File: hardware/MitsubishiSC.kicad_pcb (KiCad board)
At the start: 6 copper layers, 35 x 50 mm, 68 parts, among them J1 CN105, J2 USB_C_Receptacle_USB2.0_16P, J3 Conn_01x04, Q1 BSS138, Q2 BSS138, SW3 SPST, SW4 SPST, U1 TPS563201, U3 ESP32-C6-WROOM-1, U4 USBLC6-2SC6, U5 TLV75733PDBV

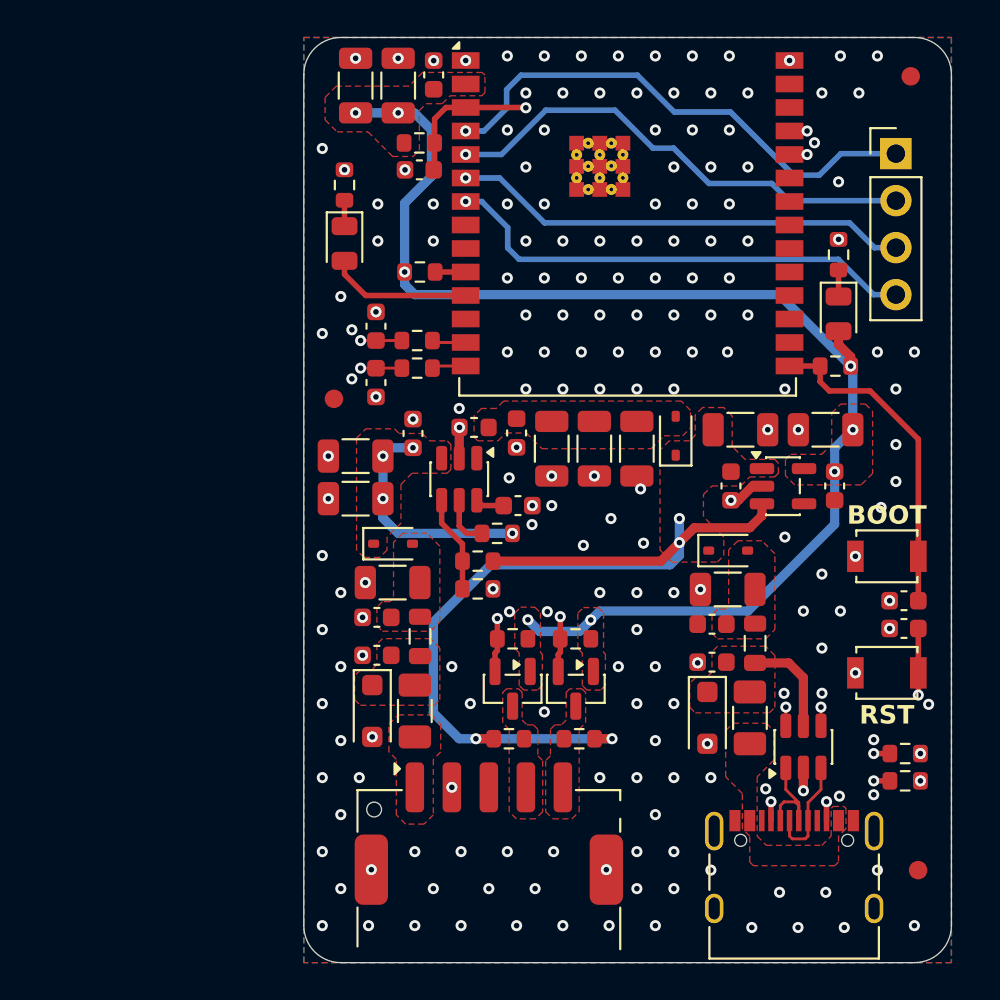
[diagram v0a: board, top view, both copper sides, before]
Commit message: feat: redesign PCB layout (#41)
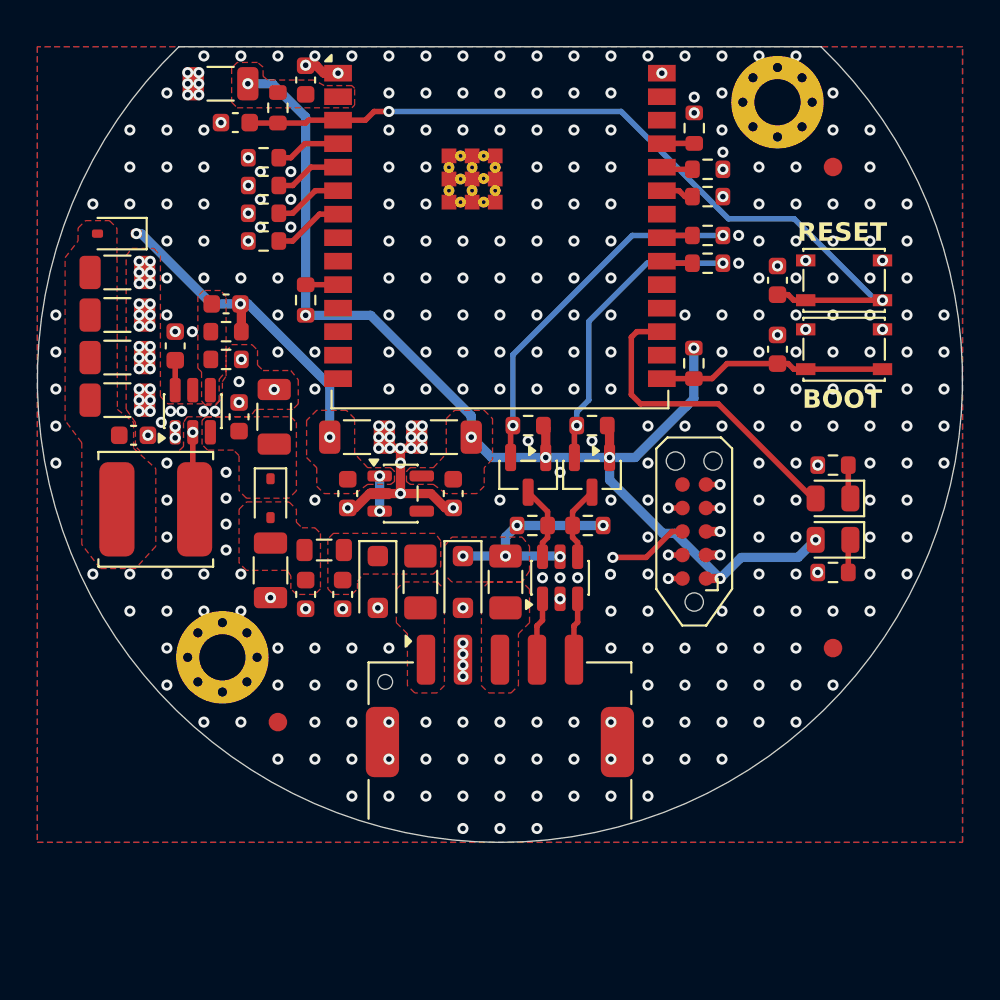
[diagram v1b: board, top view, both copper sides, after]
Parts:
- removed C22: 10uF, Capacitor_SMD:C_1206_3216Metric
- removed C23, C26: 100nF, Capacitor_SMD:C_0603_1608Metric
- removed C24, C25: NC, Capacitor_SMD:C_0603_1608Metric
- removed D7: CUS10S30, Diode_SMD:D_SOD-323
- removed D8: SMF4L5.0A, Diode_SMD:D_SOD-123F
- removed FB2: 220R@100MHz, Inductor_SMD:L_0805_2012Metric
- removed J3: Conn_01x04, Connector_PinHeader_2.54mm:PinHeader_1x04_P2.54mm_Vertical
- removed SW3, SW4: SPST, Button_Switch_SMD:SW_SPST_B3U-1000P
- removed U5: TLV75733PDBV, Package_TO_SOT_SMD:SOT-23-5
- added D6: BU, LED_SMD:LED_0805_2012Metric, F.Cu at (171.1, 104.5)
- added H1: #2, MountingHole:MountingHole_2.5mm_Pad_Via, F.Cu at (168.1, 83.1)
- added H2: #2, MountingHole:MountingHole_2.5mm_Pad_Via, F.Cu at (138.1, 113.1)
- added R17: 10kR, Resistor_SMD:R_0603_1608Metric, F.Cu at (157.8, 106.0)
- added R18: 10kR, Resistor_SMD:R_0603_1608Metric, F.Cu at (158.1, 100.6)
- added R19: 10kR, Resistor_SMD:R_0603_1608Metric, F.Cu at (171.1, 108.5)
- added R20: 10kR, Resistor_SMD:R_0603_1608Metric, F.Cu at (171.1, 102.7)
- added SW1: SPST, Button_Switch_SMD:SW_SPST_PTS810, F.Cu at (171.7, 92.7)
- added SW2: SPST, Button_Switch_SMD:SW_SPST_PTS810, F.Cu at (171.7, 96.5)
- added U2: TPS54202DDC, Package_TO_SOT_SMD:SOT-23-6, F.Cu at (136.5, 99.8)
- C11, C17, C20, C21: value 10uF -> 100nF; footprint Capacitor_SMD:C_1206_3216Metric -> Capacitor_SMD:C_0603_1608Metric
- C13, C14, C15, C19: value 100nF -> 10uF; footprint Capacitor_SMD:C_0603_1608Metric -> Capacitor_SMD:C_1206_3216Metric
- C16: value 10uF -> 68pF; footprint Capacitor_SMD:C_1206_3216Metric -> Capacitor_SMD:C_0603_1608Metric
- D1: value SMF4L12A -> CUS10S30; footprint Diode_SMD:D_SOD-123F -> Diode_SMD:D_SOD-323
- D3: value RED -> SMF4L12A; footprint LED_SMD:LED_0805_2012Metric -> Diode_SMD:D_SOD-123F
- D4: value CUS10S30 -> SMF4L5.0A; footprint Diode_SMD:D_SOD-323 -> Diode_SMD:D_SOD-123F
- D5: value BLUE -> RD
- F2: value 350mA -> 125mA
- J2: value USB_C_Receptacle_USB2.0_16P -> TC2050; footprint Connector_USB:USB_C_Receptacle_XKB_U262-16XN-4BVC11 -> Connector:Tag-Connect_TC2050-IDC-NL_2x05_P1.27mm_Vertical
- L1: value 3.3uH -> 15uH; footprint Inductor_SMD:L_0603_1608Metric -> Inductor_SMD:L_TDK_VLS6045EX_VLS6045AF
- R10: value 54.9kR -> 10kR
- R11, R12, R3, R4, R6: value 10kR -> 0R
- R13: value 10kR -> 100kR
- R14: value 5.1kR -> 13.3kR
- R15: value 5.1kR -> 10kR
- R16: value 22R -> 10kR
- R5: value 10kR -> 470R
- R7: value 22R -> 0R
- R9: value 1kR -> 0R
- U1: value TPS563201 -> ESP32-C6-WROOM-1; footprint Package_TO_SOT_SMD:SOT-23-6 -> _Custom:ESP32-C6-WROOM-1
- U3: value ESP32-C6-WROOM-1 -> TLV75733PDBV; footprint _Custom:ESP32-C6-WROOM-1 -> Package_TO_SOT_SMD:SOT-23-5
- moved FID3 48.9 mm to (141.1, 116.6)
- moved R14 43.2 mm to (138.3, 97.0)
- moved FID2 38.3 mm to (171.1, 86.6)
- moved C14 36.2 mm to (132.4, 94.6), turned to 0 degrees
- moved R3 35.7 mm to (140.3, 86.1), turned to 0 degrees
- moved C19 34.4 mm to (140.7, 108.4), turned to -90 degrees
- moved C4 33.7 mm to (135.6, 96.3), turned to 90 degrees
- moved C18 32.3 mm to (142.6, 109.7), turned to -90 degrees
- moved R1 31.4 mm to (141.1, 83.4), turned to -90 degrees
- moved R9 31.1 mm to (140.3, 90.6), turned to 0 degrees
- moved D5 30.9 mm to (171.1, 106.8), turned to 180 degrees
- moved FID1 30.1 mm to (171.1, 112.6)
- moved R4 29.7 mm to (140.3, 87.6)
- moved D1 29.3 mm to (132.4, 90.2), turned to 180 degrees
- moved D3 28.8 mm to (146.5, 109.0)
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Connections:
- C1 pad 1: +12V -> +3.3V
- C11 pad 1: +3.3V -> /SMPS_SW_5V
- C12 pad 1: +3.3V -> /SMPS_SW_5V
- C13 pad 1: /CN105_12V_FLT -> /SMPS_SW_5V
- C14 pad 1: /USB_5V_D -> /SMPS_SW_5V
- C15 pad 1: /CN105_12V_D -> /SMPS_SW_5V
- C16 pad 1: /SMPS_5V_D -> +5V
- C16 pad 2: GND -> /SMPS_FB
- C17 pad 1: /SMPS_5V_D -> /CN105_12V_FSD
- C18 pad 1: /MCU_BOOT -> /CN105_12V_FLT
- C19 pad 1: /MCU_RST -> /CN105_12V_FLT
- C2 pad 1: /SMPS_5V -> +3.3V
- C2 pad 2: /SMPS_BST -> GND
- C20 pad 1: /CN105_12V_D -> /MCU_RST
- C21 pad 1: /USB_5V_D -> /MCU_BOOT
- C3 pad 1: +12V -> /MCU_RST
- C4 pad 1: /USB_5V_FLT -> /SMPS_BOOT
- C4 pad 2: GND -> /SMPS_SW
- C6 pad 1: /SMPS_5V_D -> +12V
- D1 pad 1: /CN105_12V_FLT -> +5V
- D1 pad 2: GND -> /SMPS_SW_5V
- D2 pad 1: +5V -> +12V
- D2 pad 2: /SMPS_5V_D -> /CN105_12V_FLT
- D3 pad 1: Net-(D3-K) -> /CN105_12V_FSD
- D3 pad 2: +3.3V -> GND
- D4 pad 1: +5V -> /CN105_5V_FSD
- D4 pad 2: /USB_5V_D -> GND
- D5 pad 1: Net-(D5-K) -> /MCU_3V3_K
- D5 pad 2: /MCU_LED_STAT -> +3.3V
- F1 pad 2: /CN105_12V_FLT -> /CN105_12V_FSD
- F2 pad 1: /USB_5V -> /CN105_5V
- F2 pad 2: /USB_5V_FLT -> /CN105_5V_FSD
- FB1 pad 1: /USB_5V_FLT -> /CN105_12V_FSD
- FB1 pad 2: /USB_5V_D -> /CN105_12V_FLT
- J1 pad 3: unconnected-(J1-5V-Pad3) -> /CN105_5V
- L1 pad 1: /SMPS_5V -> /SMPS_SW
- L1 pad 2: /SMPS_5V_D -> /SMPS_SW_5V
- Q1 pad 2: /MCU_UART_RX -> /CN105_TXL
- Q1 pad 3: /CN105_TX -> /CN105_TXH
- Q2 pad 2: /MCU_UART_TX -> /CN105_RXL
- Q2 pad 3: /CN105_RX -> /CN105_RXH
- R1 pad 2: /MCU_UART_RX -> /MCU_RST
- R10 pad 1: +5V -> +3.3V
- R10 pad 2: /SMPS_FB -> /MCU_IO08
- R11 pad 1: /SMPS_FB -> /DBG_TXD
- R11 pad 2: GND -> /MCU_RX0
- R12 pad 1: +3.3V -> /MCU_TX0
- R12 pad 2: /MCU_GPIO8 -> /DBG_RXD
- R13 pad 1: +3.3V -> +5V
- R13 pad 2: /MCU_RST -> /SMPS_FB
- R14 pad 1: /USB_CC2 -> /SMPS_FB
- R15 pad 1: /USB_CC1 -> /CN105_5V_FSD
- R15 pad 2: GND -> /CN105_TXH
- R16 pad 1: /MCU_USB_D+ -> +3.3V
- R16 pad 2: /ESD_USB_D+ -> /CN105_TXL
- R2 pad 1: +5V -> +3.3V
- R2 pad 2: /CN105_TX -> /MCU_BOOT
- R3 pad 1: +5V -> /DBG_JTMS
- R3 pad 2: /CN105_RX -> /MCU_MTMS
- R4 pad 1: +3.3V -> /MCU_MTDI
- R4 pad 2: /MCU_UART_TX -> /DBG_JTDI
- R5 pad 1: +12V -> /CN105_RXL
- R5 pad 2: /SMPS_EN -> /MCU_TX1
- R6 pad 1: +3.3V -> /MCU_RX1
- R6 pad 2: /MCU_BOOT -> /CN105_TXL
- R7 pad 1: /ESD_USB_D- -> /MCU_MTCK
- R7 pad 2: /MCU_USB_D- -> /DBG_JTCK
- R8 pad 1: Net-(D5-K) -> /MCU_IO15
- R9 pad 1: Net-(D3-K) -> /DBG_JTDO
- R9 pad 2: GND -> /MCU_MTDO
- U1 pad 2: /SMPS_5V -> +3.3V
- U1 pad 3: +12V -> /MCU_RST
- U1 pad 4: /SMPS_FB -> /MCU_MTMS
- U1 pad 5: /SMPS_EN -> /MCU_MTDI
- U1 pad 6: /SMPS_BST -> /MCU_MTCK
- U3 pad 1: GND -> +5V
- U3 pad 2: +3.3V -> GND
- U3 pad 3: /MCU_RST -> +5V
- U3 pad 4: /MCU_GPIO4 -> unconnected-(U3-NC-Pad4)
- U3 pad 5: /MCU_GPIO5 -> +3.3V
- U4 pad 1: /USB_D- -> /CN105_TX
- U4 pad 3: /USB_D+ -> /CN105_RX
- U4 pad 4: /ESD_USB_D+ -> /CN105_RXH
- U4 pad 5: /USB_5V_FLT -> /CN105_5V_FSD
- U4 pad 6: /ESD_USB_D- -> /CN105_TXH
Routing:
- net /ESD_USB_D-: track 44.3 -> 0.00 mm, vias 2 -> 0
- net /ESD_USB_D+: track 43.7 -> 0.00 mm, vias 2 -> 0
- net /DBG_JTMS: track 0.00 -> 39.1 mm, vias 0 -> 2
- net /MCU_UART_TX: track 38.5 -> 0.00 mm, vias 2 -> 0
- net /MCU_UART_RX: track 37.0 -> 0.00 mm, vias 2 -> 0
- net /DBG_JTCK: track 0.00 -> 31.5 mm, vias 0 -> 2
- net /DBG_JTDO: track 0.00 -> 31.1 mm, vias 0 -> 2
- net /DBG_JTDI: track 0.00 -> 30.9 mm, vias 0 -> 2
- net +5V: track 50.0 -> 20.1 mm, vias 4 -> 5
- net /MCU_GPIO4: track 27.8 -> 0.00 mm, vias 1 -> 0
- net /MCU_GPIO5: track 26.3 -> 0.00 mm, vias 1 -> 0
- net /MCU_GPIO7: track 26.0 -> 0.00 mm, vias 1 -> 0
- net /MCU_GPIO6: track 24.8 -> 0.00 mm, vias 1 -> 0
- net /DBG_TXD: track 0.00 -> 24.6 mm, vias 0 -> 2
- net /DBG_RXD: track 0.00 -> 22.4 mm, vias 0 -> 2
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- added copper zone on F.Cu, net /CN105_12V_FSD
- added copper zone on F.Cu, net /CN105_5V
- added copper zone on F.Cu, net /CN105_5V_FSD
- added copper zone on F.Cu, net /SMPS_FB
- added copper zone on F.Cu, net /SMPS_SW_5V
- removed copper zone on F.Cu, net /CN105_12V_D
- removed copper zone on F.Cu, net /CN105_RX
- removed copper zone on F.Cu, net /CN105_TX
- removed copper zone on F.Cu, net /SMPS_5V_D
- removed copper zone on F.Cu, net /USB_5V
- removed copper zone on F.Cu, net /USB_5V_D
- removed copper zone on F.Cu, net /USB_5V_FLT
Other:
- board size 35 x 50 mm -> 50 x 43 mm
- board text added: "RESET"
- board text removed: "RST"
